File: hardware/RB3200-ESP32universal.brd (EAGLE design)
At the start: 73.7 x 44.5 mm, 102 parts, among them IC1 FT232R, IC2 7805, T1 BC337, T2 BC337, U1 ESP-WROOM-32, U2 UM18533, X1 USB-MICRO-B-BOTTOM

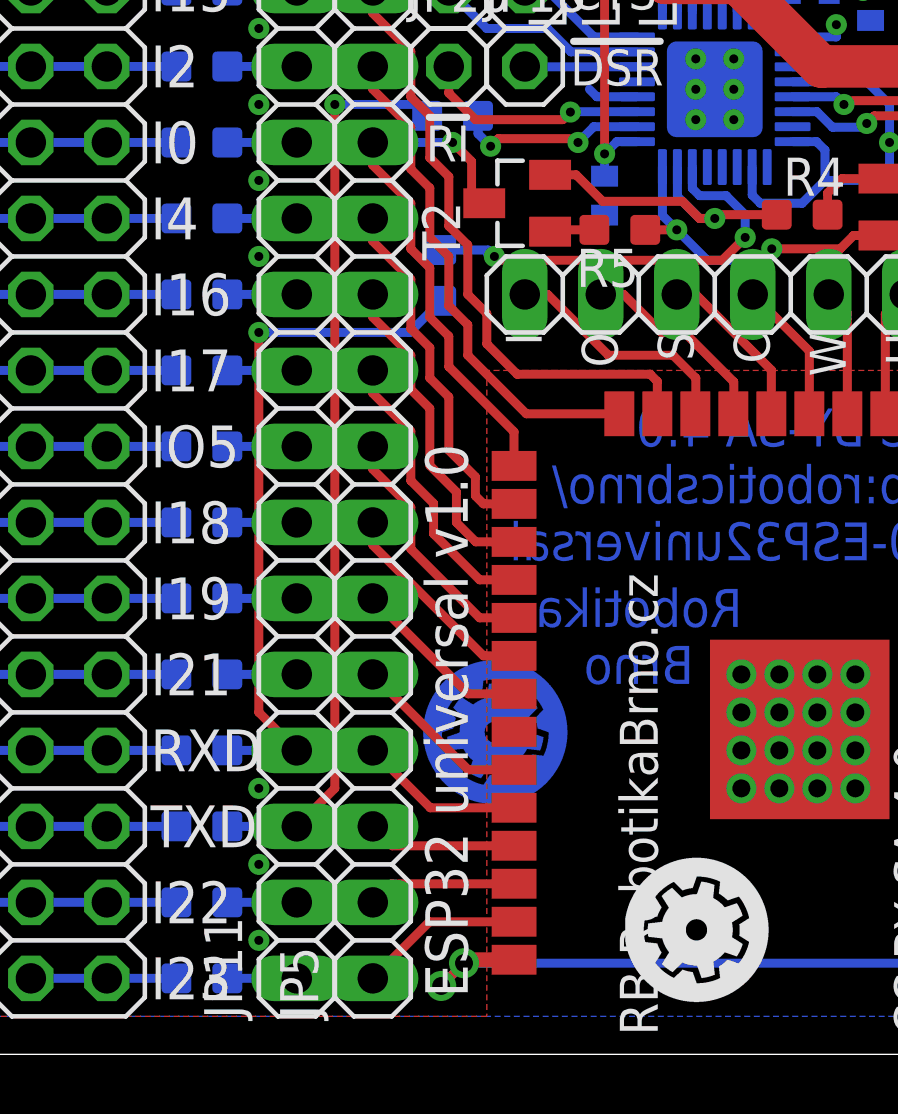
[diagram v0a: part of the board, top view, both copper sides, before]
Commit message: Add information text about license and authors
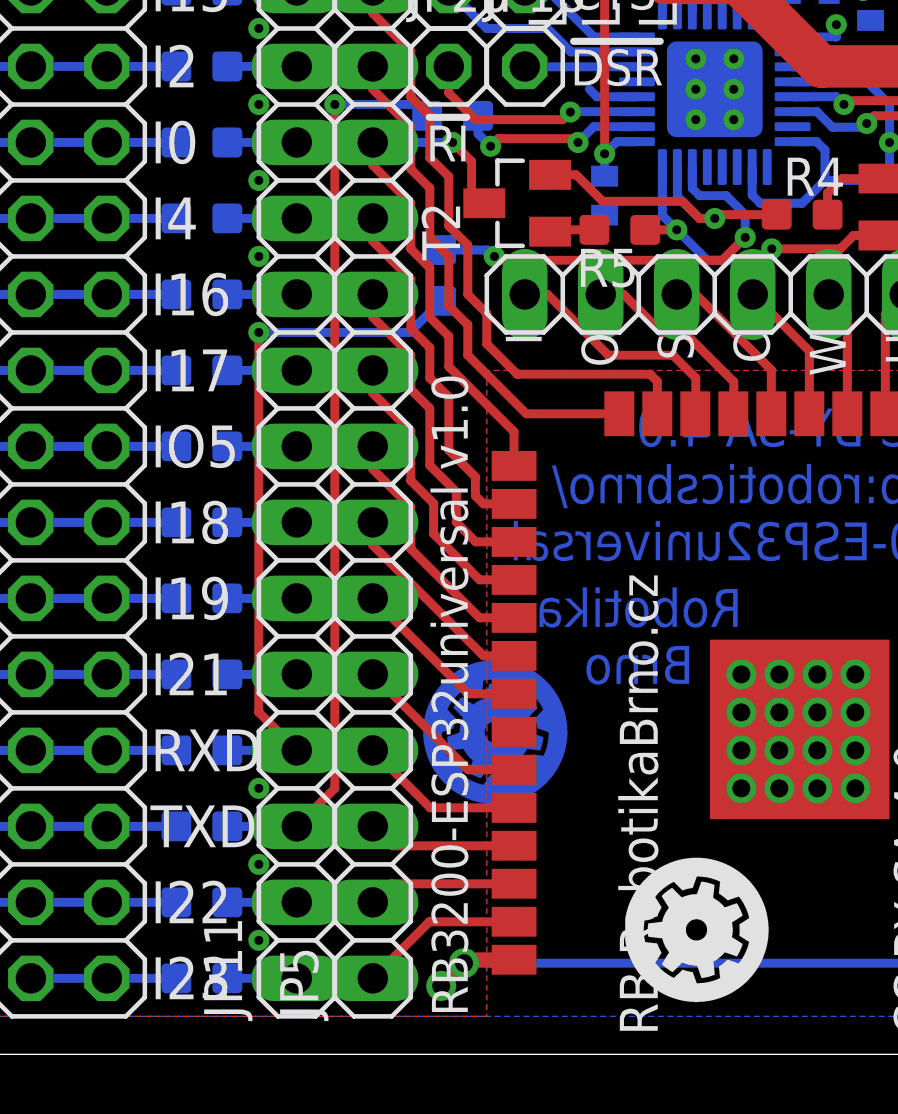
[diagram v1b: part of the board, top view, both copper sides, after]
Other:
- board text added: "RB3200-ESP32universal v1.0"
- board text added: "Released under the Creative Commons Attribution-ShareAlike 4.0 License https://creativecommons.org/licenses/by-sa/4.0/ Designed by: JM & JP & JS & JV & RobotikaBrno RB3200-ESP32universal https://github.com/RoboticsBrno/RB3200-ESP32universal RobotikaBrno.cz Robotarna"
- board text removed: "ESP32 universal v1.0"
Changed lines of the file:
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@@
 <circle x="2.54" y="41.91" radius="2.54" width="0.3" layer="41"/>
 <circle x="71.12" y="41.91" radius="2.54" width="0.3" layer="41"/>
-<text x="26.035" y="1.905" size="1.4224" layer="102" font="vector" ratio="20" rot="R90">ESP32 universal v1.0</text>
+<text x="26.035" y="1.27" size="1.2" layer="102" font="vector" ratio="20" rot="R90">RB3200-ESP32universal v1.0</text>
 <text x="15.4305" y="32.3215" size="1.4" layer="102" font="vector" ratio="20">I2</text>
 <text x="15.4305" y="29.7815" size="1.4" layer="102" font="vector" ratio="20">I0</text>
@@
 <text x="28.702" y="41.91" size="1.2" layer="102" font="vector" ratio="20" rot="R270">CBS2</text>
 <text x="26.924" y="41.91" size="1.2" layer="102" font="vector" ratio="20" rot="R270">CBS4</text>
-<wire x1="-0.635" y1="0.635" x2="73.025" y2="0.635" width="0" layer="103"/>
+<wire x1="0" y1="0.635" x2="73.66" y2="0.635" width="0" layer="103"/>
 <text x="0.508" y="38.608" size="1.6764" layer="102" font="vector" ratio="16" rot="R270">5
 3
@@
 <text x="31.75" y="13.97" size="1.27" layer="16" font="vector" ratio="16" rot="MR180" align="center">Robotika
 Brno</text>
+<text x="36.83" y="-18.415" size="1.778" layer="48" font="vector" align="center">Released under the Creative Commons Attribution-ShareAlike 4.0 License
+https://creativecommons.org/licenses/by-sa/4.0/
+Designed by: JM &amp; JP &amp; JS &amp; JV &amp; RobotikaBrno
+RB3200-ESP32universal
+https://github.com/RoboticsBrno/RB3200-ESP32universal
+RobotikaBrno.cz
+Robotarna</text>
 </plain>
 <attributes>

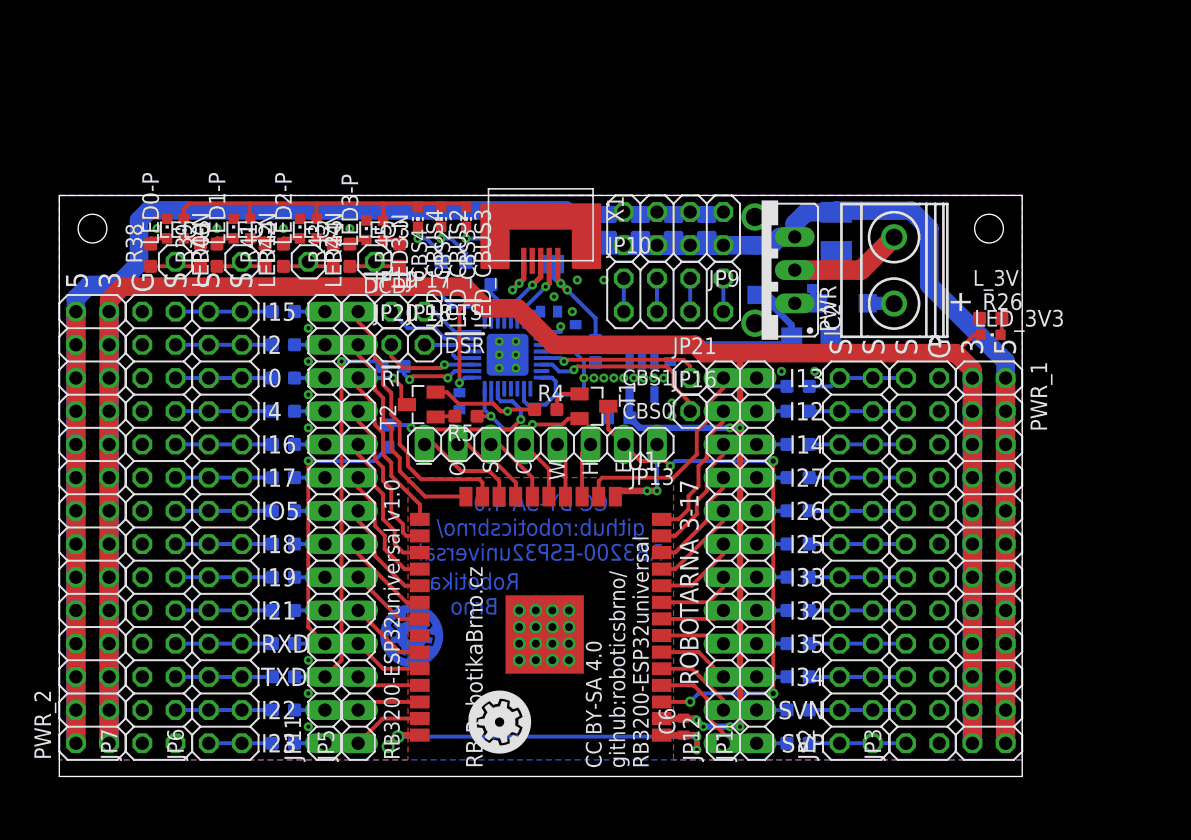
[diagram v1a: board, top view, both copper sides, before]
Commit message: Publish version 2.0 of RB3200-ESP32universal and level_shifter DPS
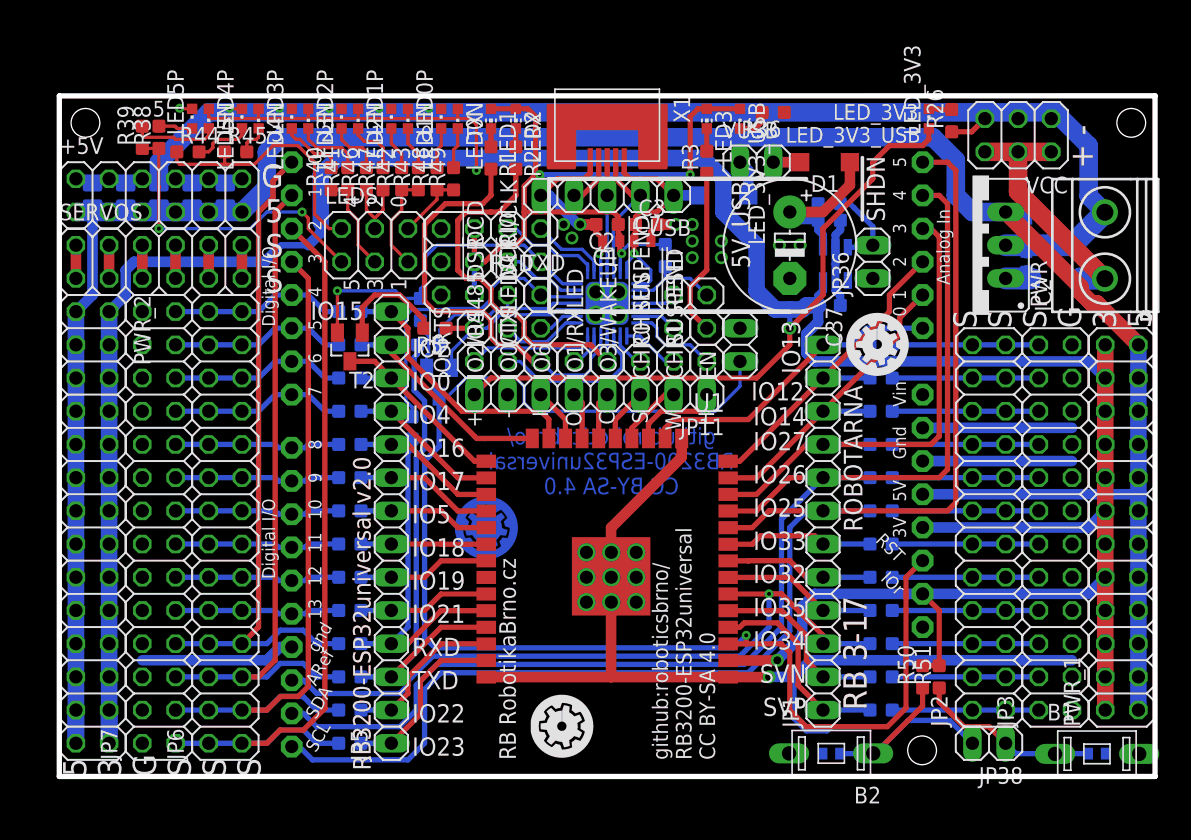
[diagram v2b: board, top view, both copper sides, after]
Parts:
- removed C12: 4u7, rcl_upravena:C0805
- removed C13: 100n, rcl_upravena:C0402
- removed C14: 22u/16V, rcl_upravena:SMC_B
- removed D3: skl34, diode:SOD123
- removed IC1: FT232R, ftdichip_upravena:QFN32_LONG_PADS
- removed JP10, JP9: (no value), pinhead:2X04
- removed JP12: (no value), pinhead:1X12
- removed JP13: (no value), pinhead:1X08
- removed JP16, JP17, JP18, JP19, JP20, JP21, LED0: (no value), pinhead:1X01
- removed LED0-N, LED0-P, LED1-N, LED1-P, LED2-N, LED2-P, LED3-N, LED3-P: green, led:CHIPLED_0603
- removed LED_CBUS2, LED_CBUS3, LED_CBUS4: yellow, led:CHIP-LED0603
- added !CTS, !DCD, !DSR, !DTR, !RESET, !RTS, !SUSPEND, CHR0, CHR1, CHREN, IO0/TXLED, IO1/RXLED, IO2/RS485, IO3/WAKEUP, IO4, IO5, IO6, RI/CLK, RXD, SUSPEND, TXD: PINH1X01, pinhead_smd:1X01
- added +5V, SERVOS: (no value), pinhead:2X06
- added B1, B2: TACTM-35N-F, TACTM-35N-F:TACTM-35N-F
- added C20, C21: 100n/16V, rcl_upravena:C0402
- added C37: 330u/16V, rcl_upravena:E5-10,5
- added C67, C70: 4u7/16V, rcl_upravena:C0805
- added D5: skl34, diode:SOD123
- added EN, JP36, JP38, VUSB: (no value), pinhead:1X02
- added IC3: CP2102N-28, CP2102N:QFN28-PAD
- added LED0N, LED1N, LED2N, LED3N, LED4N, LED5N: red, led:CHIPLED_0603
- added LED0P, LED1P, LED2P, LED3P, LED4P, LED5P, LED_3V3_USB: green, led:CHIPLED_0603
- added LEDS, VCC, VCCIO: (no value), pinhead:2X03
- added R35, R50, R51: 10k, rcl_upravena:R0603
- added R36, R46, R48: 470R, rcl_upravena:R0603
- added R37: 100k, rcl_upravena:R0603
- added R47, R49: 680R, rcl_upravena:R0603
- added U3: ARDUINOR3-BPLACE, adafruit:ARDUINOR3-BPLACE
- added USB: (no value), pinhead:1X05
- C1, C6, C7: value 100n -> 100n/16V
- C10, C3, C5, C9: value 4u7 -> 4u7/16V
- C11: value 4u7 -> 100n/16V; device rcl_upravena:C0805 -> rcl_upravena:C0402
- C2, C4: value 100n -> 4u7/16V; device rcl_upravena:C0402 -> rcl_upravena:C0603
- C8: value 22u/16V -> 4u7/16V; device rcl_upravena:SMC_B -> rcl_upravena:C0805
- D1: value (none) -> skl34; device diode:MINIMELF -> diode:SOD123
- JP11: device pinhead:1X14 -> pinhead:1X08
- LED1, LED2, LED3: value (none) -> yellow; device pinhead:1X01 -> led:CHIP-LED0603
- R1, R2, R26, R3, R38, R40, R42, R44: value 180R -> 470R
- R39, R41, R43, R45: value 180R -> 680R
- moved C8 49.4 mm to (10.2, 44.5), turned to 90 degrees
- moved C10 42.0 mm to (5.08, 44.5), turned to 90 degrees
- moved C11 41.4 mm to (59.1, 1.75), turned to 180 degrees
- moved C9 36.9 mm to (7.62, 44.5), turned to 90 degrees
- moved C6 31.7 mm to (79.4, 1.75), flipped to the bottom, turned to 0 degrees
- moved LED3 27.7 mm to (49.5, 50.3), turned to 180 degrees
- moved JP11 22.7 mm to (40.6, 29.2), turned to 180 degrees
- moved R3 22.0 mm to (49.5, 47.0), flipped to the top, turned to 90 degrees
- moved LED1 22.0 mm to (33.0, 50.3), turned to 180 degrees
- moved D1 21.7 mm to (58.6, 47.0), flipped to the top, turned to 180 degrees
- moved LED2 19.3 mm to (34.9, 50.3), turned to 180 degrees
- moved C5 18.3 mm to (58.9, 36.0), turned to 180 degrees
- moved LED_3V3 17.2 mm to (66.5, 50.3), turned to 0 degrees
- moved U2 17.2 mm to (59.4, 39.2)
- moved C1 16.9 mm to (42.2, 41.0), flipped to the top, turned to 180 degrees
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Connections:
- net LED renamed LED_3V3
- removed net !CTS: IC1.8, JP17.1
- removed net !DCD: IC1.7, JP19.1
- removed net !DSR: IC1.6, JP18.1
- removed net !RI: IC1.3, JP20.1
- removed net 3V3_FTDI: C2.1, IC1.16
- removed net 5V->3V3: C14.+, C4.1, D2.C, U2.P$1, U2.P$3
- removed net CBUS0: IC1.22, JP16.1
- removed net CBUS1: IC1.21, JP21.1
- removed net CBUS2: IC1.10, R1.2
- removed net CBUS2_LED: LED_CBUS2.C, R1.1
- removed net CBUS3: IC1.11, R2.2
- removed net CBUS3_LED: LED_CBUS3.C, R2.1
- removed net CBUS4: IC1.9, R3.2
- removed net CBUS4_LED: LED_CBUS4.C, R3.1
- removed net LED0: LED0.1, R38.1, R39.1
- removed net LED0-N: LED0-N.C, R39.2
- removed net LED0-P: LED0-P.A, R38.2
- removed net LED1: LED1.1, R40.1, R41.1
- removed net LED1-N: LED1-N.C, R41.2
- removed net LED1-P: LED1-P.A, R40.2
- removed net LED2: LED2.1, R42.1, R43.1
- removed net LED2-N: LED2-N.C, R43.2
- removed net LED2-P: LED2-P.A, R42.2
- removed net LED3-N: LED3-N.C, R45.2
- removed net LED3-P: LED3-P.A, R44.2
- removed net N$10: JP2.5, JP2.6, JP3.6, R7.1
- removed net N$11: JP2.3, JP2.4, JP3.4, R6.1
- removed net N$12: JP2.1, JP2.2, JP3.2, R19.1
- removed net N$13: JP6.25, JP6.26, JP7.25, R32.1
- removed net N$14: JP6.23, JP6.24, JP7.23, R31.1
- removed net N$15: JP6.21, JP6.22, JP7.21, R30.1
- removed net N$16: JP6.19, JP6.20, JP7.19, R29.1
- removed net N$17: JP6.17, JP6.18, JP7.17, R28.1
- removed net N$18: JP6.15, JP6.16, JP7.15, R27.1
- removed net N$19: JP6.13, JP6.14, JP7.13, R25.1
- removed net N$20: JP6.11, JP6.12, JP7.11, R24.1
- removed net N$21: JP6.10, JP6.9, JP7.9, R23.1
- removed net N$23: JP6.5, JP6.6, JP7.5, R21.1
- removed net N$24: JP6.3, JP6.4, JP7.3, R20.1
- removed net N$25: JP10.1, JP10.2
- removed net N$26: JP6.1, JP6.2, JP7.1, R22.1
- removed net N$27: JP6.7, JP6.8, JP7.7, R33.1
- removed net N$28: JP6.27, JP6.28, JP7.27, R34.1
- removed net N$29: JP10.3, JP10.4
- removed net N$30: JP10.5, JP10.6
- removed net N$5: JP2.15, JP2.16, JP3.16, R14.1
- removed net N$6: JP2.13, JP2.14, JP3.14, R13.1
- removed net N$7: JP2.11, JP2.12, JP3.12, R10.1
- removed net N$8: JP2.10, JP2.9, JP3.10, R9.1
- removed net N$9: JP2.7, JP2.8, JP3.8, R8.1
- removed net USBDM: IC1.15, X1.2
- removed net USBDP: IC1.14, X1.3
- new net !RESET: !RESET.1, IC3.9, R35.1
- new net !SHDN: JP36.2, R37.2, U2.P$3
- new net !SUSPEND: !SUSPEND.1, IC3.11
- new net 3V3_IN: C37.+, C4.1, D1.C, R37.1, U2.P$1
- new net 5V_USB: D2.C, VUSB.1
- new net BTN0: B1.P$4, C6.2, JP38.1, R51.1
- new net BTN1: B2.P$4, C11.2, JP38.2, R50.1
- new net CHR0: CHR0.1, IC3.15
- new net CHR1: CHR1.1, IC3.14
- new net CHREN: CHREN.1, IC3.13
- new net CLK/!RI: IC3.2, RI/CLK.1
- new net DCD: !DCD.1, IC3.1
- new net DM: IC3.5, USB.2, X1.2
- new net DP: IC3.4, USB.3, X1.3
- new net DSR: !DSR.1, IC3.27
- new net IO0_!RST!_: JP5.12, R31.2, T2.3, U1.25
- new net IO12_: JP1.11, R17.2, U1.14, U3.A2
- new net IO13_: JP1.12, R18.2, U1.16, U3.A0
- new net IO14_: JP1.10, R16.2, U1.13, U3.A1
- new net IO15_: JP5.14, R34.2, U1.23
- new net IO16_: JP5.10, R29.2, U1.27
- new net IO17_: JP5.9, R28.2, U1.28
- new net IO18_: JP5.7, R25.2, U1.30
- new net IO19_: JP5.6, R24.2, U1.31
- new net IO21_: JP5.5, R23.2, U1.33
- new net IO22_: JP5.2, R20.2, U1.36
- new net IO23_: JP5.1, R22.2, U1.37
- new net IO25_: JP1.7, R13.2, U1.10, U3.A5, U3.SCL
- new net IO26_: JP1.8, R14.2, U1.11, U3.A4, U3.SDA
- new net IO27_: JP1.9, R15.2, U1.12, U3.A3
- new net IO2_: JP5.13, R32.2, U1.24
- new net IO32_: JP1.5, R9.2, U1.8
- new net IO33_: JP1.6, R10.2, U1.9
- new net IO34_: JP1.3, R7.2, U1.6, U3.AREF
- new net IO35_: JP1.4, R8.2, U1.7
- new net IO4_: JP5.11, R30.2, U1.26
- new net IO5_: JP5.8, R27.2, U1.29
- new net LED0N: LED0N.C, R49.2
- new net LED0P: LED0P.A, R48.2
- new net LED1N: LED1N.C, R43.2
- new net LED1P: LED1P.A, R42.2
- new net LED2N: LED2N.C, R47.2
- new net LED2P: LED2P.A, R46.2
- new net LED3N: LED3N.C, R41.2
- new net LED3P: LED3P.A, R40.2
- new net LED4N: LED4N.C, R45.2
- new net LED4P: LED4P.A, R44.2
- new net LED5N: LED5N.C, R39.2
- new net LED5P: LED5P.A, R38.2
- new net LED_0: LEDS.6, R48.1, R49.1
- new net LED_1: LEDS.5, R42.1, R43.1
- new net LED_2: LEDS.4, R46.1, R47.1
- new net LED_3: LEDS.3, R40.1, R41.1
- new net LED_3V3_USB: LED_3V3_USB.C, R36.2
- new net LED_4: LEDS.2, R44.1, R45.1
- new net LED_5: LEDS.1, R38.1, R39.1
- new net N$32: SERVOS.3, SERVOS.4
- new net N$34: SERVOS.7, SERVOS.8
- new net N$36: SERVOS.11, SERVOS.12
- new net RX-LED: LED2.C, R2.1
- new net RXD0_: JP5.4, R11.2, R33.2, U1.34
- new net RX_LED: IC3.18, IO1/RXLED.1, R2.2
- new net SENSOR_VN_: JP1.2, R6.2, U1.5
- new net SENSOR_VP_: JP1.1, R19.2, U1.4
- new net SUSPEND: IC3.12, R3.1, SUSPEND.1
- new net TX-LED: LED1.C, R1.1
- new net TXD0_: JP5.3, R12.2, R21.2, U1.35
- new net TX_LED: IC3.19, IO0/TXLED.1, R1.2
- new net USBID: USB.4, X1.4
- new net USBIO3_RS485: IC3.17, IO2/RS485.1
- new net USBIO3_WAKEUP: IC3.16, IO3/WAKEUP.1
- new net USBIO4: IC3.22, IO4.1
- new net USBIO5: IC3.21, IO5.1
- new net USBIO6: IC3.20, IO6.1
- new net VCCIO: C1.1, C2.1, IC3.6, LED1.A, LED2.A, LED3.A, LED_3V3_USB.A, R35.2, VCCIO.2, VCCIO.4, VCCIO.6
- new net VUSB: C3.1, C7.1, D2.A, IC3.7, IC3.8, USB.1, X1.1
- net !DTR: now also !DTR.1, IC3.28; no longer IC1.31
- net !RTS: now also !RTS.1, IC3.24; no longer IC1.32
- net +3V3: now also JP11.8, LED0N.A, LED1N.A, LED2N.A, LED3N.A, LED4N.A, LED5N.A, PWR_1.10, PWR_1.12, PWR_1.14, PWR_1.16, PWR_1.18, PWR_1.2, PWR_1.20, PWR_1.22, PWR_1.24, PWR_1.4, PWR_1.6, PWR_1.8, PWR_2.10, PWR_2.12, PWR_2.14, PWR_2.16, PWR_2.18, PWR_2.2, PWR_2.20, PWR_2.22, PWR_2.24, PWR_2.26, PWR_2.28, PWR_2.4, PWR_2.6, PWR_2.8, R50.2, R51.2, U3.3V, U3.IOREF; no longer C1.1, C6.2, IC1.1, LED0-N.A, LED1-N.A, LED2-N.A, LED3-N.A, LED_CBUS2.A, LED_CBUS3.A, LED_CBUS4.A, PWR_1.1, PWR_1.11, PWR_1.13, PWR_1.15, PWR_1.17, PWR_1.19, PWR_1.21, PWR_1.23, PWR_1.3, PWR_1.5, PWR_1.7, PWR_1.9, PWR_2.1, PWR_2.11, PWR_2.13, PWR_2.15, PWR_2.17, PWR_2.19, PWR_2.21, PWR_2.23, PWR_2.25, PWR_2.27, PWR_2.3, PWR_2.5, PWR_2.7, PWR_2.9
- net +5V: now also +5V.1, +5V.11, +5V.3, +5V.5, +5V.7, +5V.9, C10.1, C20.1, C67.1, C70.1, C8.1, C9.1, D1.A, PWR_1.1, PWR_1.11, PWR_1.13, PWR_1.15, PWR_1.17, PWR_1.19, PWR_1.21, PWR_1.23, PWR_1.3, PWR_1.5, PWR_1.7, PWR_1.9, PWR_2.1, PWR_2.11, PWR_2.13, PWR_2.15, PWR_2.17, PWR_2.19, PWR_2.21, PWR_2.23, PWR_2.25, PWR_2.27, PWR_2.3, PWR_2.5, PWR_2.7, PWR_2.9, U3.5V, VUSB.2; no longer C10.2, C11.2, C12.2, C8.+, C9.2, D1.C, D2.A, JP9.2, JP9.4, JP9.6, JP9.8, PWR_1.10, PWR_1.12, PWR_1.14, PWR_1.16, PWR_1.18, PWR_1.2, PWR_1.20, PWR_1.22, PWR_1.24, PWR_1.4, PWR_1.6, PWR_1.8, PWR_2.10, PWR_2.12, PWR_2.14, PWR_2.16, PWR_2.18, PWR_2.2, PWR_2.20, PWR_2.22, PWR_2.24, PWR_2.26, PWR_2.28, PWR_2.4, PWR_2.6, PWR_2.8
- net EN: now also EN.1, U3.RESET; no longer JP13.2
- net GND: now also +5V.10, +5V.12, +5V.2, +5V.4, +5V.6, +5V.8, B1.P$2, B2.P$2, C10.2, C20.2, C21.2, C37.-, C67.2, C70.2, C8.2, C9.2, EN.2, IC3.3, IC3.PAD, JP11.7, JP36.1, LED0P.C, LED1P.C, LED2P.C, LED3P.C, LED4P.C, LED5P.C, R36.1, U3.GND, U3.GND1, U3.GND2, USB.5, VCC.1, VCC.3, VCC.5, VCCIO.1, VCCIO.3, VCCIO.5; no longer C10.1, C12.1, C13.2, C14.-, C8.-, C9.1, IC1.17, IC1.20, IC1.24, IC1.26, IC1.4, JP13.1, JP9.1, JP9.3, JP9.5, JP9.7, LED0-P.C, LED1-P.C, LED2-P.C, LED3-P.C
- net IO0_!RST: now also JP6.23, JP6.24, JP7.23, R31.1, U3.D6; no longer JP11.12, JP5.12, R31.2, T2.3, U1.25
- net IO12: now also JP2.21, JP2.22, JP3.22, R17.1; no longer JP1.11, JP12.11, R17.2, U1.14
- net IO13: now also JP2.23, JP2.24, JP3.24, R18.1; no longer JP1.12, JP12.12, R18.2, U1.16
- net IO14: now also JP2.19, JP2.20, JP3.20, R16.1; no longer JP1.10, JP12.10, R16.2, U1.13
- net IO15: now also JP6.27, JP6.28, JP7.27, R34.1, U3.D4; no longer JP11.14, JP5.14, R34.2, U1.23
- net IO16: now also JP6.19, JP6.20, JP7.19, R29.1, U3.D8; no longer JP11.10, JP5.10, R29.2, U1.27
- net IO17: now also JP6.17, JP6.18, JP7.17, R28.1, U3.D9; no longer JP11.9, JP5.9, R28.2, U1.28
- net IO18: now also JP6.13, JP6.14, JP7.13, R25.1, U3.D11; no longer JP11.7, JP5.7, R25.2, U1.30
- net IO19: now also JP6.11, JP6.12, JP7.11, R24.1, U3.D12; no longer JP11.6, JP5.6, R24.2, U1.31
- net IO2: now also JP6.25, JP6.26, JP7.25, R32.1, U3.D5; no longer JP11.13, JP5.13, R32.2, U1.24
- net IO21: now also JP6.10, JP6.9, JP7.9, R23.1, U3.D13; no longer JP11.5, JP5.5, R23.2, U1.33
- net IO22: now also JP6.3, JP6.4, JP7.3, R20.1, U3.D3; no longer JP11.2, JP5.2, R20.2, U1.36
- net IO23: now also JP6.1, JP6.2, JP7.1, R22.1, U3.D2; no longer JP11.1, JP5.1, R22.2, U1.37
- net IO25: now also JP2.13, JP2.14, JP3.14, R13.1; no longer JP1.7, JP12.7, R13.2, U1.10
- net IO26: now also JP2.15, JP2.16, JP3.16, R14.1; no longer JP1.8, JP12.8, R14.2, U1.11
- net IO27: now also JP2.17, JP2.18, JP3.18, R15.1; no longer JP1.9, JP12.9, R15.2, U1.12
- net IO32: now also JP2.10, JP2.9, JP3.10, R9.1; no longer JP1.5, JP12.5, R9.2, U1.8
- net IO33: now also JP2.11, JP2.12, JP3.12, R10.1; no longer JP1.6, JP12.6, R10.2, U1.9
- net IO34: now also JP2.5, JP2.6, JP3.6, R7.1; no longer JP1.3, JP12.3, R7.2, U1.6
- net IO35: now also JP2.7, JP2.8, JP3.8, R8.1; no longer JP1.4, JP12.4, R8.2, U1.7
- net IO4: now also JP6.21, JP6.22, JP7.21, R30.1, U3.D7; no longer JP11.11, JP5.11, R30.2, U1.26
- net IO5: now also JP6.15, JP6.16, JP7.15, R27.1, U3.D10; no longer JP11.8, JP5.8, R27.2, U1.29
- net N$1: now also U3.RESERVED; no longer JP2.23, JP2.24, JP3.24, R18.1
- net N$2: now also !CTS.1, IC3.23; no longer JP2.21, JP2.22, JP3.22, R17.1
- net N$3: now also U3.VIN; no longer JP2.19, JP2.20, JP3.20, R16.1
- net N$31: now also SERVOS.1, SERVOS.2; no longer JP10.7, JP10.8
- net N$33: now also SERVOS.5, SERVOS.6; no longer C3.1, C7.1, D1.A, IC1.19, X1.1
- net N$35: now also SERVOS.10, SERVOS.9; no longer LED3.1, R44.1, R45.1
- net N$4: now also LED3.C, R3.2; no longer JP2.17, JP2.18, JP3.18, R15.1
- net NC-CS: now also JP11.3; no longer JP13.5
- net NC-HOLD: now also JP11.1; no longer JP13.3
- net NC-MISO: now also JP11.6; no longer JP13.8
- net NC-MOSI: now also JP11.5; no longer JP13.7
- net NC-SCK: now also JP11.4; no longer JP13.6
- net NC-WP: now also JP11.2; no longer JP13.4
- net RXD: now also IC3.25, RXD.1; no longer IC1.2
- net RXD0: now also JP6.7, JP6.8, JP7.7, R33.1, U3.D0; no longer JP11.4, JP5.4, R11.2, R33.2, U1.34
- net SENSOR_VN: now also JP2.3, JP2.4, JP3.4, R6.1; no longer JP1.2, JP12.2, R6.2, U1.5
- net SENSOR_VP: now also JP2.1, JP2.2, JP3.2, R19.1; no longer JP1.1, JP12.1, R19.2, U1.4
- net TXD: now also IC3.26, TXD.1; no longer IC1.30
- net TXD0: now also JP6.5, JP6.6, JP7.5, R21.1, U3.D1; no longer JP11.3, JP5.3, R12.2, R21.2, U1.35
- net VCC: now also D5.A, VCC.2, VCC.4, VCC.6; no longer D3.A
- net VCC->5V: now also C21.1, D5.C; no longer C13.1, D3.C
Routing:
- net GND: track 70.4 -> 233.2 mm, vias 61 -> 32
- net IO25_: track 0.00 -> 106.0 mm
- net IO26_: track 0.00 -> 99.1 mm
- net EN: track 42.3 -> 104.2 mm, vias 4 -> 1
- net VCCIO: track 0.00 -> 58.6 mm, vias 0 -> 3
- net IO34_: track 0.00 -> 54.6 mm, vias 0 -> 1
- net IO23: track 10.4 -> 58.5 mm
- net IO22: track 9.84 -> 52.2 mm
- net IO27_: track 0.00 -> 38.4 mm
- net TXD0_: track 0.00 -> 38.0 mm
- net TX_LED: track 0.00 -> 32.8 mm
- net RX_LED: track 0.00 -> 28.6 mm
- net RXD0_: track 0.00 -> 26.9 mm
- net IO12_: track 0.00 -> 25.5 mm
- net IO14_: track 0.00 -> 25.0 mm
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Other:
- board size 73.7 x 44.5 mm -> 83.8 x 52.1 mm
- board text added: "!SHDN"
- board text added: "+ -"
- board text added: "0"
- board text added: "1"
- board text added: "2"
- board text added: "3"
- board text added: "4"
- board text added: "4 2 0"
- board text added: "5"
- board text added: "5 3 1"
- board text added: "5V_USB"
- board text added: "G 5 S S"
- board text added: "IO0"
- board text added: "IO12"
- board text added: "IO13"
- board text added: "IO14"
- board text added: "IO15"
- board text added: "IO16"
- board text added: "IO17"
- board text added: "IO18"
- board text added: "IO19"
- board text added: "IO2"
- board text added: "IO21"
- board text added: "IO22"
- board text added: "IO23"
- board text added: "IO25"
- board text added: "IO26"
- board text added: "IO27"
- board text added: "IO32"
- board text added: "IO33"
- board text added: "IO34"
- board text added: "IO35"
- board text added: "IO4"
- board text added: "LED_3V3"
- board text added: "LED_3V3_USB"
- board text added: "RB 3-17"
- board text added: "RB3200-ESP32universal v2.0"
- board text added: "ROBOTARNA"
- board text added: "RX"
- board text added: "TX"
- board text added: "github:roboticsbrno/ RB3200-ESP32universal CC BY-SA 4.0"
- board text removed: "!CTS"
- board text removed: "!DCD"
- board text removed: "!DSR"
- board text removed: "!RI"
- board text removed: "CBS0"
- board text removed: "CBS1"
- board text removed: "CBS2"
- board text removed: "CBS3"
- board text removed: "CBS4"
- board text removed: "CC BY-SA 4.0 github:roboticsbrno/ RB3200-ESP32universal"
- board text removed: "E"
- board text removed: "I0"
- board text removed: "I12"
- board text removed: "I13"
- board text removed: "I14"
- board text removed: "I15"
- board text removed: "I16"
- board text removed: "I17"
- board text removed: "I18"
- board text removed: "I19"
- board text removed: "I2"
- board text removed: "I21"
- board text removed: "I22"
- board text removed: "I23"
- board text removed: "I25"
- board text removed: "I26"
- board text removed: "I27"
- board text removed: "I32"
- board text removed: "I33"
- board text removed: "I34"
- board text removed: "I35"
- board text removed: "I4"
- board text removed: "L_3V"
- board text removed: "RB3200-ESP32universal v1.0"
- board text removed: "ROBOTARNA 3-17"
- board text removed: "Robotika Brno"
